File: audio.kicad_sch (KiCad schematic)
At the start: 10 parts, among them IC1 MAX98357AETE+T, J3 i2s_mic, J6 Speaker, J7 Micro_SD_Card, U3 DFR0299

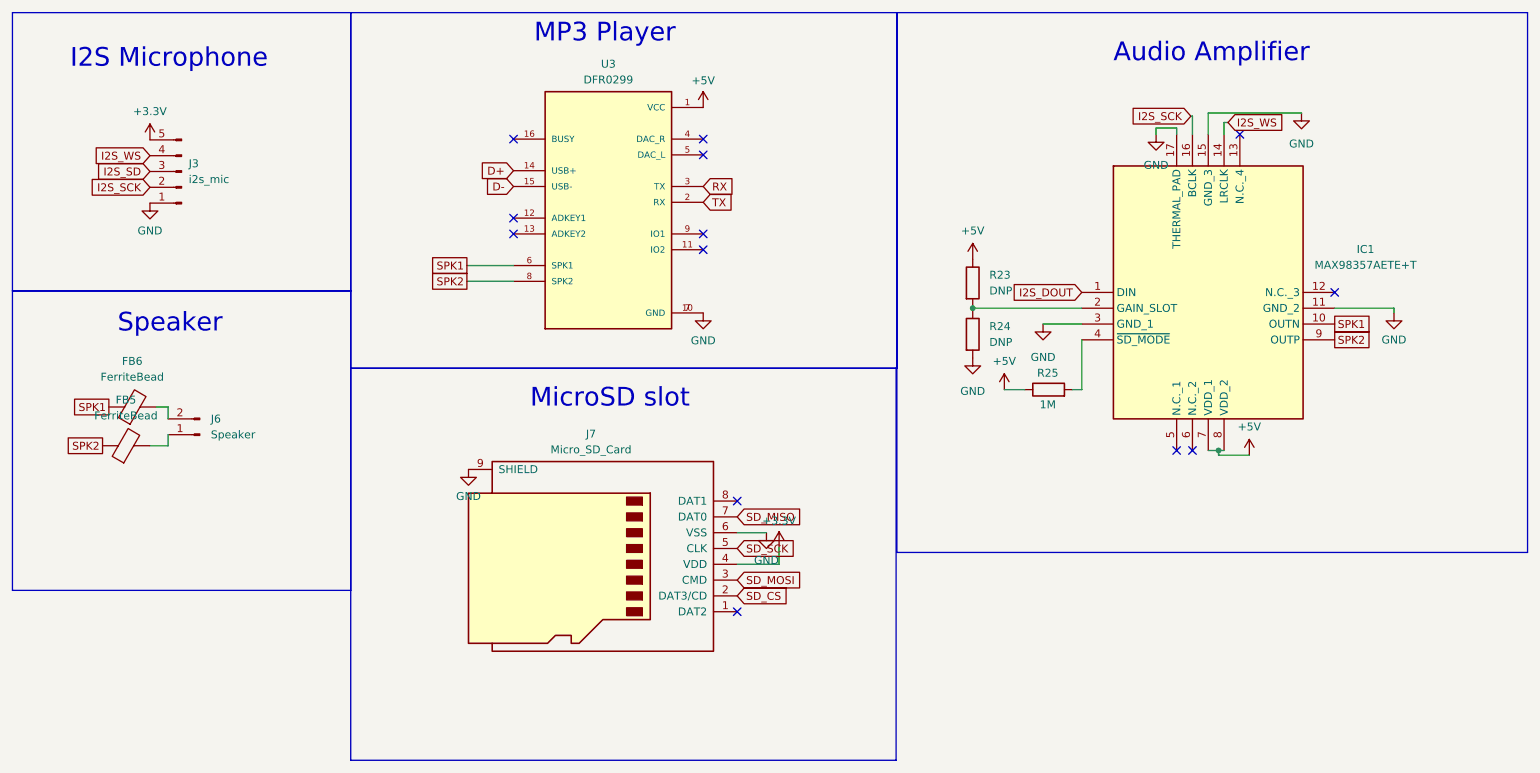
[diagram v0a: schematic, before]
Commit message: -add some changes to power section and display
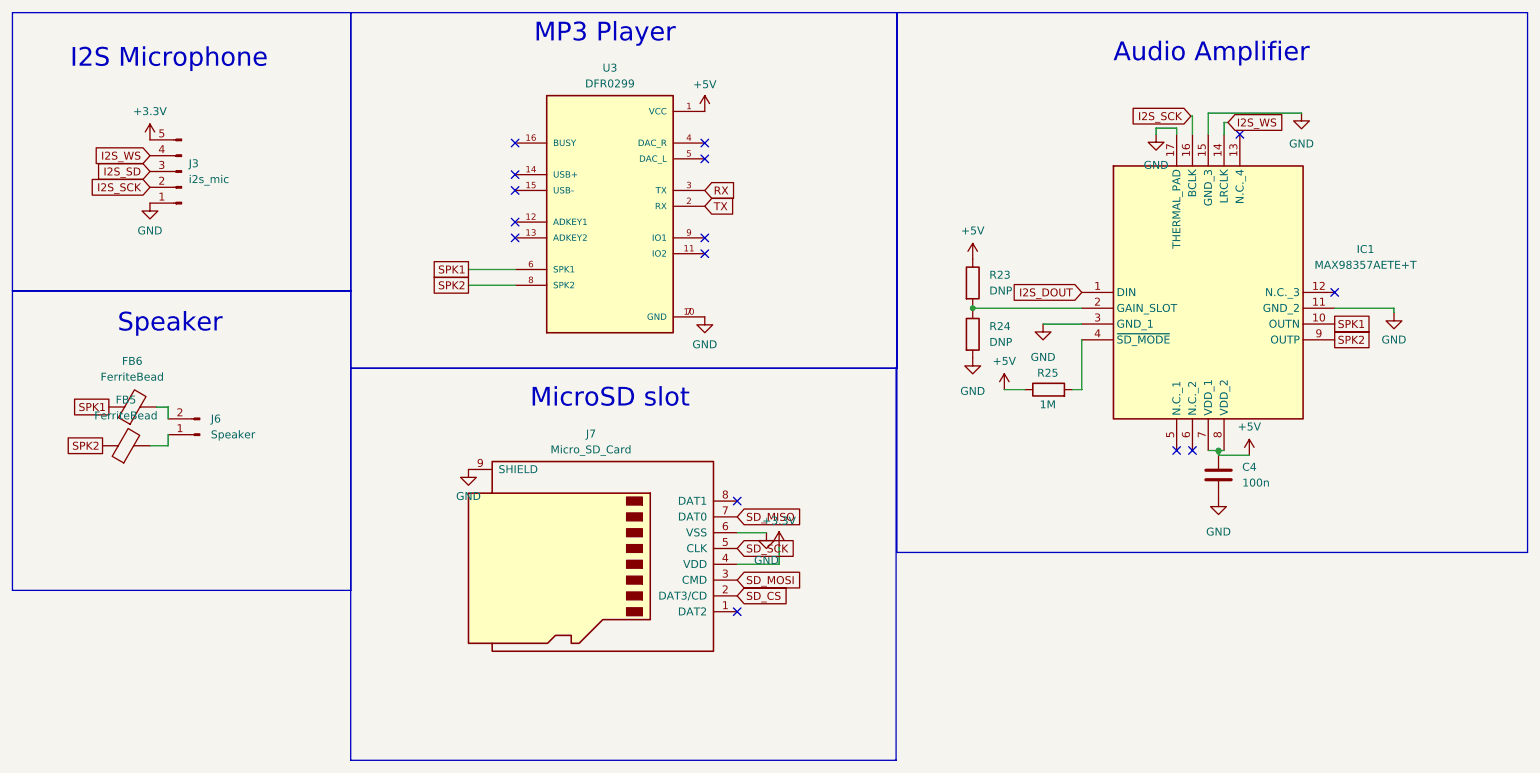
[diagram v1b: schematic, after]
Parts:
- added C4: 100n, Capacitor_SMD:C_0603_1608Metric_Pad1.08x0.95mm_HandSolder, symbol Device:C
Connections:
- net +5V: now also C4.1
- net GND: now also C4.2
- net D+: no longer names the net of U3.14 (USB+)
- net D-: no longer names the net of U3.15 (USB-)
- no-connect marks 13 -> 15
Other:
- moved on the sheet: U3

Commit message: -add end revision
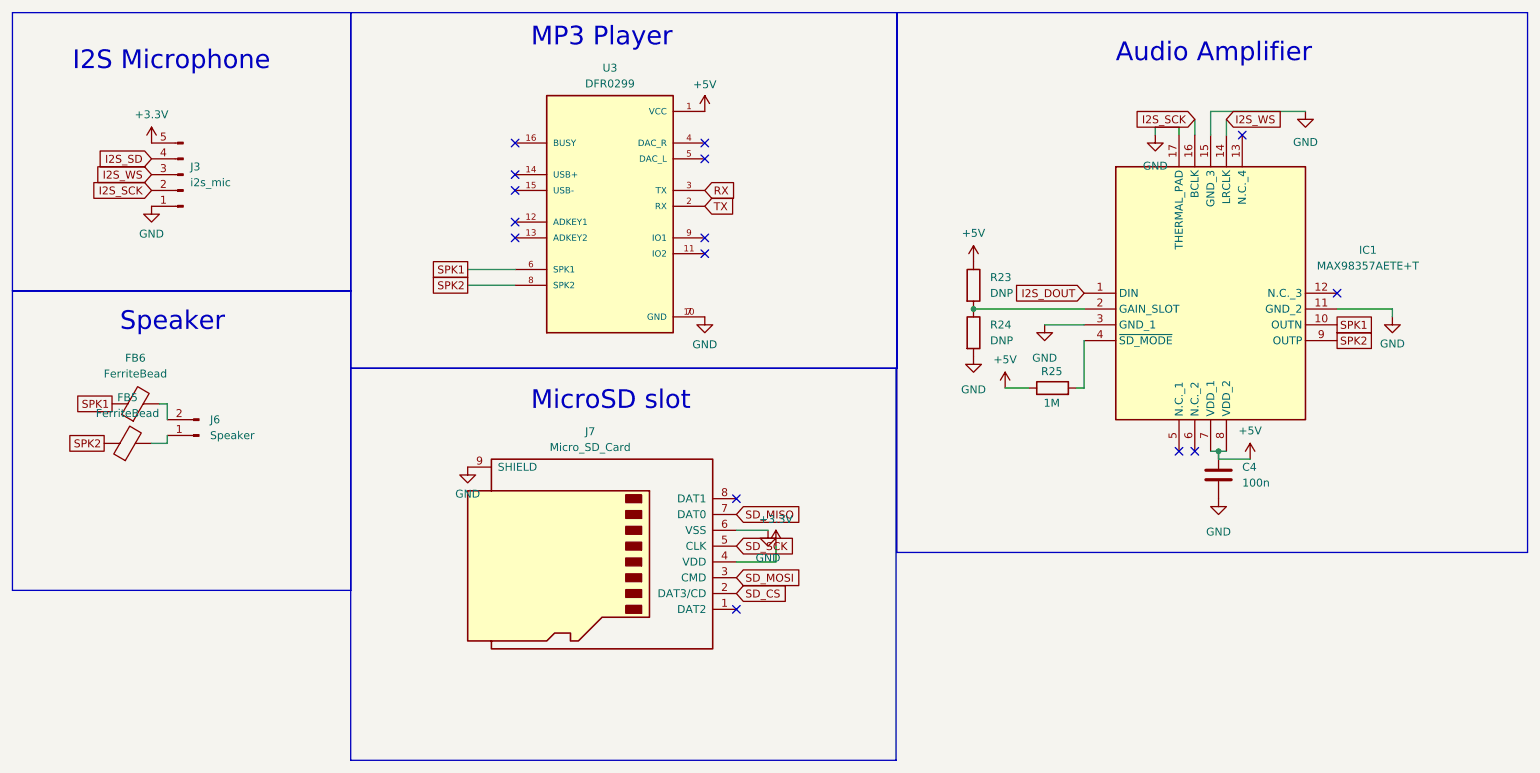
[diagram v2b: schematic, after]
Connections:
- net I2S_SD: now also J3.4 (Pin_4); no longer J3.3 (Pin_3)
- net I2S_WS: now also J3.3 (Pin_3); no longer J3.4 (Pin_4)
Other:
- moved on the sheet: FB6, J3, R25
